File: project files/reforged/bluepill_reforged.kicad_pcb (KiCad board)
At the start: 2 copper layers, 53.3 x 22.9 mm, 40 parts, among them J1 USB_C_Receptacle_USB2.0, J2 Left Castellation, J3 STDC14, J4 Right Castellation, SW1 Boot0, SW2 Reset, U1 AMS1117-3.3, U2 STM32F103C8Tx, Y1 8Mhz,TSX-3225, Y2 MC-306, 32768Hz

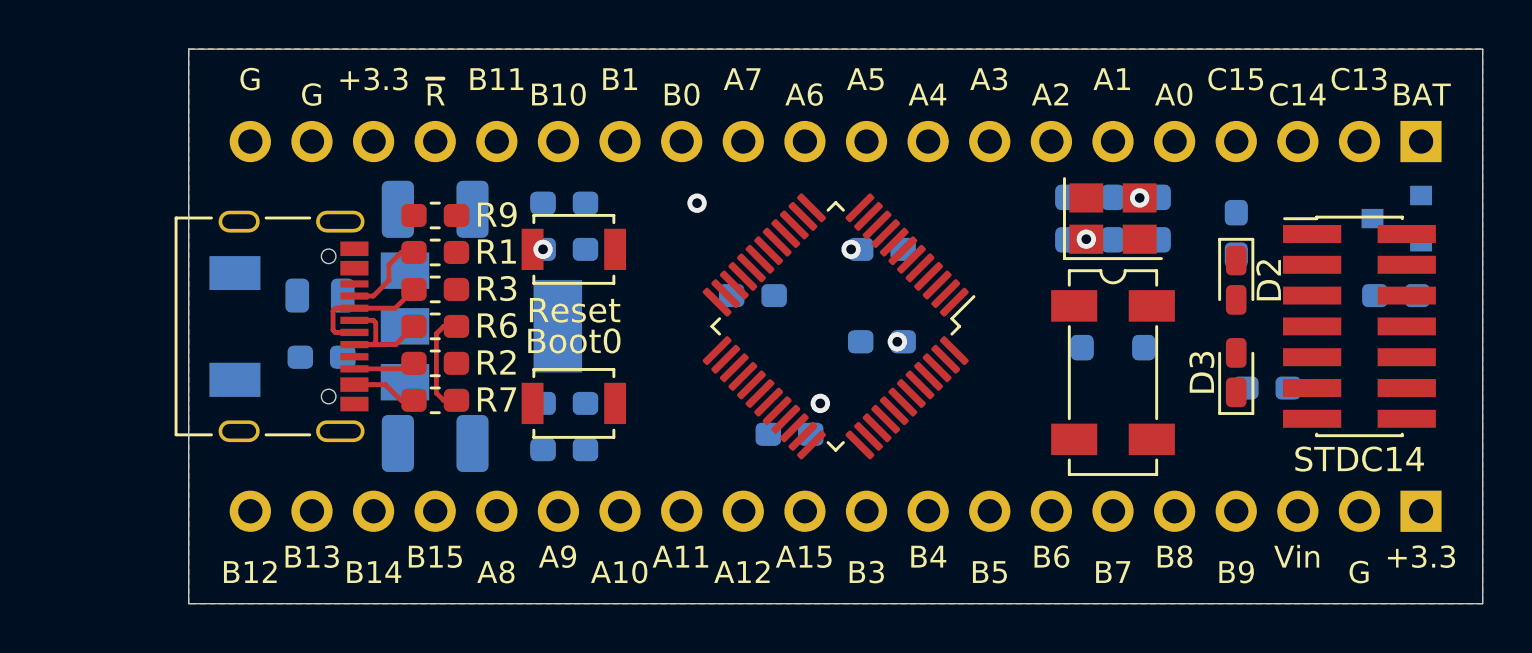
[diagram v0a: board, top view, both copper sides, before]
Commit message: rearranged
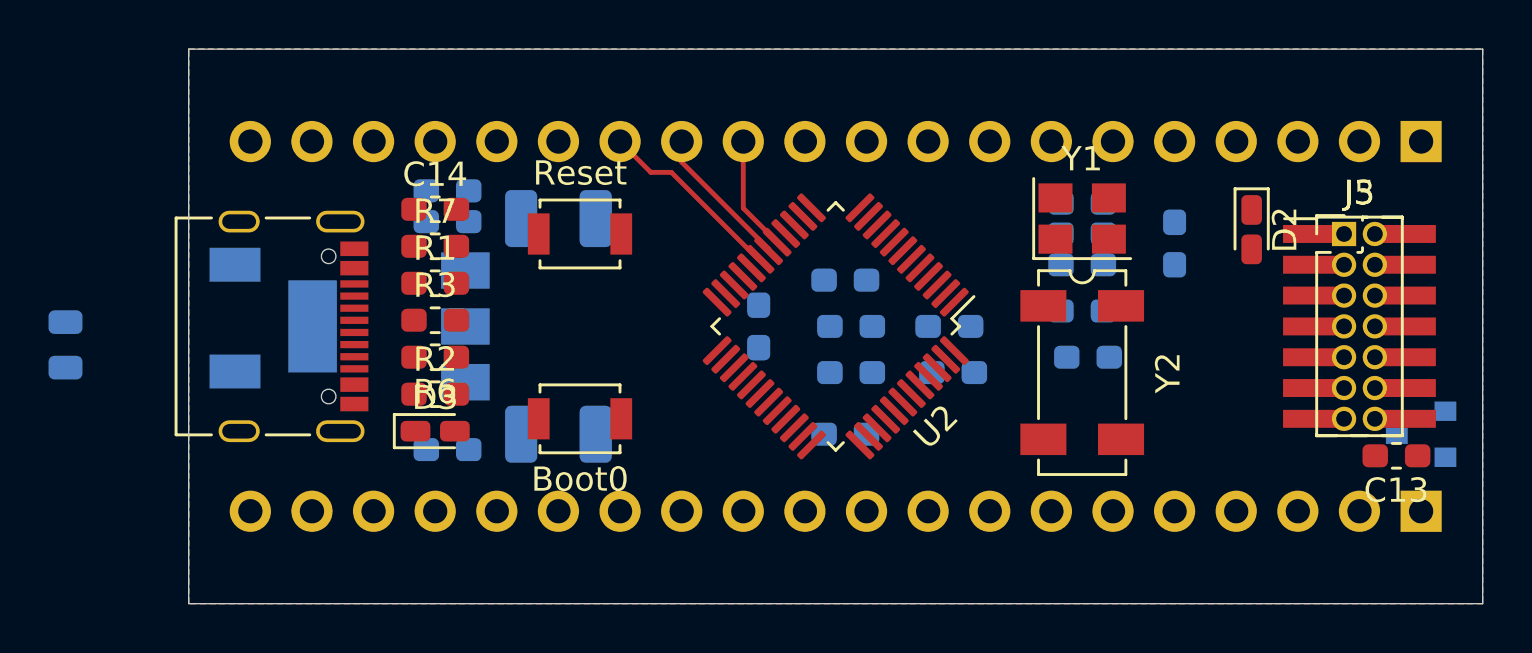
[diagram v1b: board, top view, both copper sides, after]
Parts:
- added J5: STDC14, Connector_PinHeader_1.27mm:PinHeader_2x07_P1.27mm_Vertical, F.Cu at (174.6, 134.6)
- C13, C14: moved to F.Cu
- R9: moved to B.Cu
- Y1: value 8Mhz,TSX-3225 -> 8MHz; footprint Crystal:Crystal_SMD_3225-4Pin_3.2x2.5mm -> Crystal:Crystal_SMD_TXC_7M-4Pin_3.2x2.5mm
- moved R11 33.9 mm to (137.7, 143.5), turned to 0 degrees
- moved D3 33.1 mm to (137.2, 142.7), turned to 0 degrees
- moved C13 27.3 mm to (176.8, 143.8)
- moved C9 18.5 mm to (158.4, 138.4)
- moved C3 12.9 mm to (154.3, 138.4)
- moved R4 11.9 mm to (154.3, 140.3)
- moved F1 10.7 mm to (121.9, 139.2), turned to 90 degrees
- moved C1 10.6 mm to (142.2, 142.9)
- moved C2 10.6 mm to (142.2, 134.0)
- moved R5 9.49 mm to (150.5, 138.4), turned to 90 degrees
- moved D4 8.95 mm to (177.8, 142.9)
- moved C11 7.77 mm to (154.1, 142.9)
- moved C14 7.69 mm to (137.2, 133.6)
- moved C12 6.75 mm to (154.1, 136.5), turned to 0 degrees
- moved R7 6.35 mm to (137.2, 135.1)
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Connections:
- J1 pad A8: Net-(J1-PadA8) -> (no net)
- J1 pad B8: Net-(J1-PadB8) -> (no net)
- J3 pad 1: Net-(J3-Pad1) -> (no net)
- J3 pad 10: Net-(J3-Pad10) -> (no net)
- J3 pad 2: Net-(J3-Pad2) -> (no net)
- J3 pad 9: Net-(J3-Pad9) -> (no net)
- Y2 pad 2: Net-(Y2-Pad2) -> (no net)
- Y2 pad 3: Net-(Y2-Pad3) -> (no net)
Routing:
- net PB1: track 0.00 -> 7.78 mm
- net PB0: track 0.00 -> 5.98 mm
- net D-: track 5.41 -> 0.00 mm
- net D+: track 5.41 -> 0.00 mm
- net PA7: track 0.00 -> 4.72 mm
- net PA12: track 4.35 -> 0.00 mm
- net Net-(J1-PadA5): track 3.58 -> 0.00 mm
- net VBUS: track 2.73 -> 0.00 mm
- net Net-(J1-PadB5): track 2.55 -> 0.00 mm
- net OSCOUT: vias 1 -> 0
- net OSCIN: vias 1 -> 0
- net NRST: vias 1 -> 0
- net BOOT1: vias 1 -> 0
- net +3V3: vias 3 -> 0
- added copper zone on B.Cu, net GNDD
- added copper zone on F.Cu, net GNDD
- removed copper zone on B.Cu, net GNDREF
- removed copper zone on F.Cu, net GNDREF
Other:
- net class Default: via_dia 0.8 -> 0.5; via_drill 0.4 -> 0.3
- board text removed: "+3.3"
- board text removed: "A0"
- board text removed: "A1"
- board text removed: "A10"
- board text removed: "A11"
- board text removed: "A12"
- board text removed: "A15"
- board text removed: "A2"
- board text removed: "A3"
- board text removed: "A4"
- board text removed: "A5"
- board text removed: "A6"
- board text removed: "A7"
- board text removed: "A8"
- board text removed: "A9"
- board text removed: "B0"
- board text removed: "B1"
- board text removed: "B10"
- board text removed: "B11"
- board text removed: "B12"
- board text removed: "B13"
- board text removed: "B14"
- board text removed: "B15"
- board text removed: "B3"
- board text removed: "B4"
- board text removed: "B5"
- board text removed: "B6"
- board text removed: "B7"
- board text removed: "B8"
- board text removed: "B9"
- board text removed: "BAT"
- board text removed: "C13"
- board text removed: "C14"
- board text removed: "C15"
- board text removed: "G"
- board text removed: "Vin"
- board text removed: "~R"

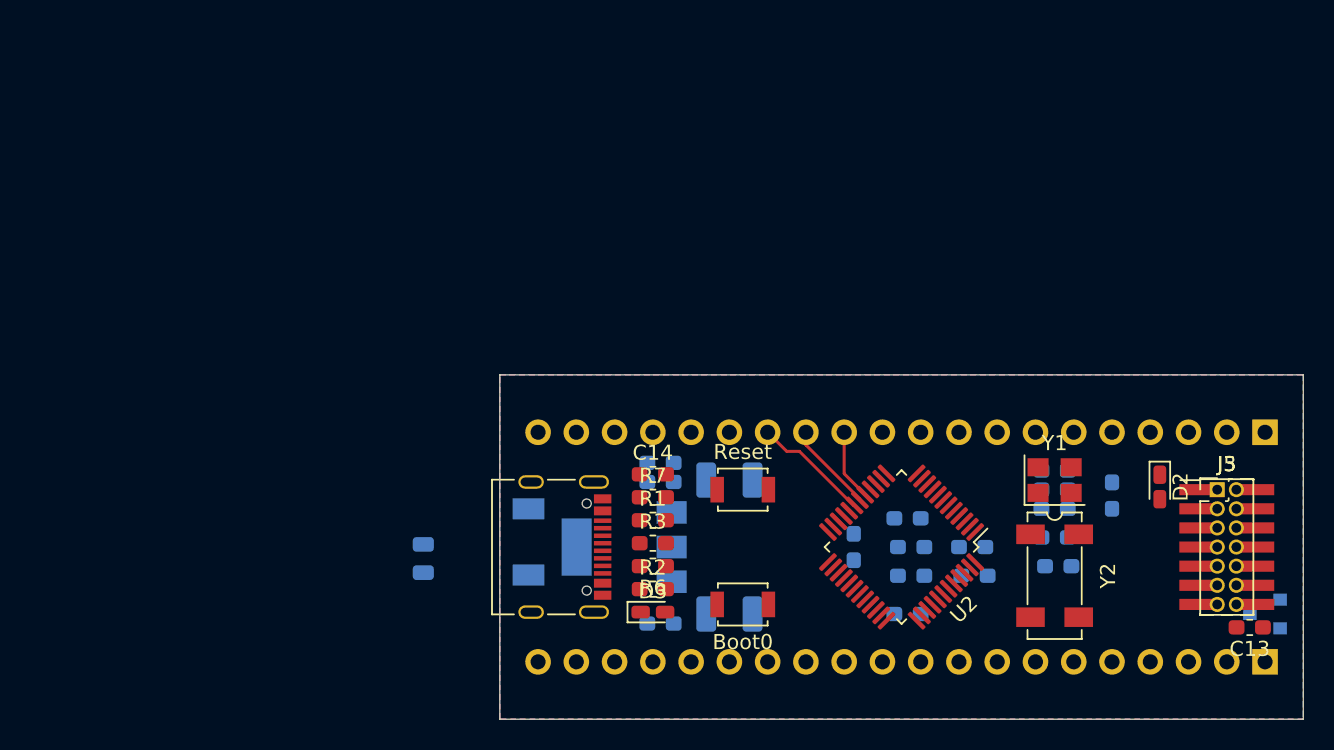
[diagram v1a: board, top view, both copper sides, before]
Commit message: edits
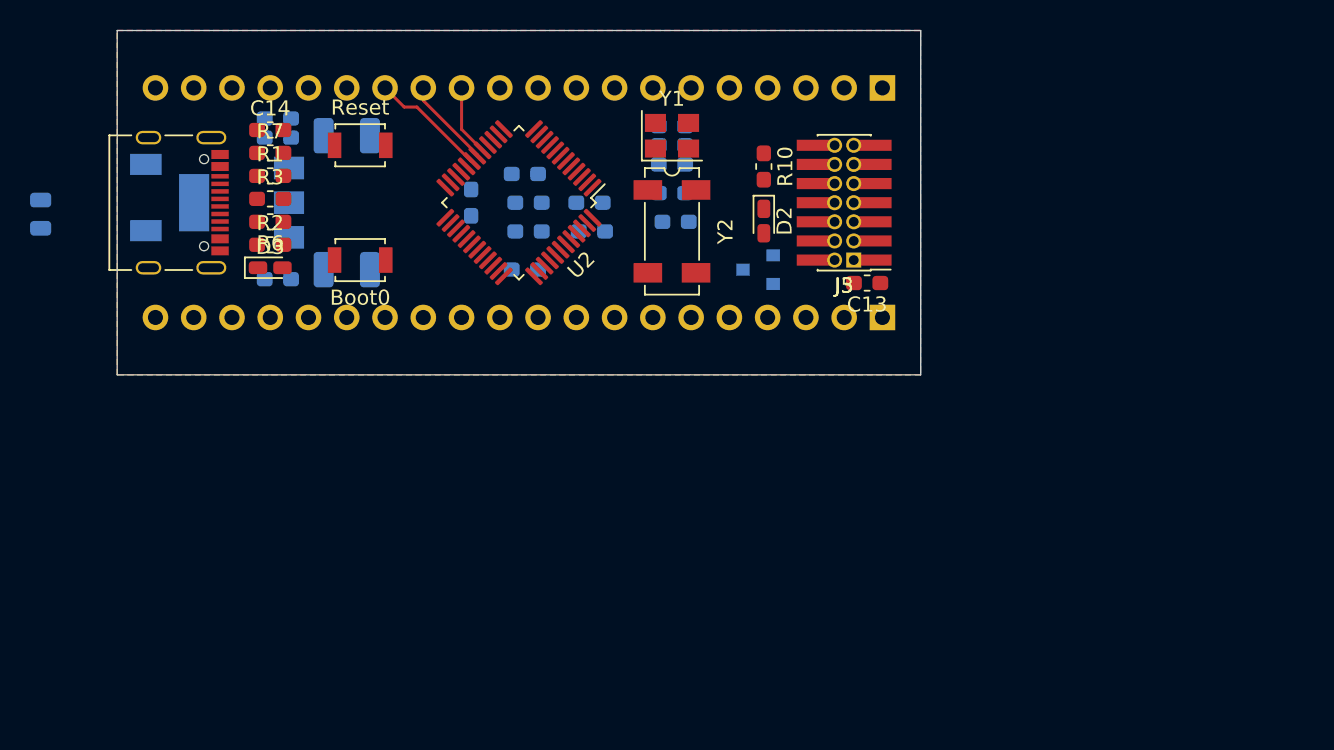
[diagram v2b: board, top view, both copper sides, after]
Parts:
- R10: moved to F.Cu
- moved D4 40.7 mm to (144.1, 120.0)
- moved C13 34.2 mm to (151.4, 120.9)
- moved C2 34.2 mm to (116.8, 111.1)
- moved C3 34.2 mm to (128.9, 115.6)
- moved F1 34.2 mm to (96.5, 116.3)
- moved J1 34.2 mm to (105.9, 115.6)
- moved J2 34.2 mm to (152.4, 123.2)
- moved R4 34.2 mm to (128.9, 117.5)
- moved R5 34.2 mm to (125.1, 115.6)
- moved R9 34.2 mm to (112.3, 110.0)
- moved Y1 34.2 mm to (138.4, 111.1)
- moved Y2 34.2 mm to (138.4, 117.5)
- moved C1 34.2 mm to (116.8, 120.0)
- moved C11 34.2 mm to (128.7, 120.0)
- moved C12 34.2 mm to (128.7, 113.7)
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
